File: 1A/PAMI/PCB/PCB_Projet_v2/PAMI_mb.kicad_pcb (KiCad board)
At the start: 4 copper layers, 66.5 x 58.4 mm, 107 parts, among them J1 Conn_02x20_Odd_Even, J10 Conn_01x04, J11 Conn_01x04, J12 Conn_01x04, J13 Conn_01x04, J2 Conn_01x03, J3 Conn_ST_STDC14, J4 Battery, J5 Charge, J6 Stop, J8 173010542, J9 Conn_01x04, SW1 SW_Push_SPDT, SW2 RotaryEncoder_Switch, SW3 SW_Push, SW4 SW_Push, SW5 SW_Push, SW6 SW_Push, U1 STM32G431KBTx, U2 LT1076CR-PBF, U3 AZ1117CH2-3.3TRG1, U4 TMC2225-SA-T, U5 TMC2225-SA-T

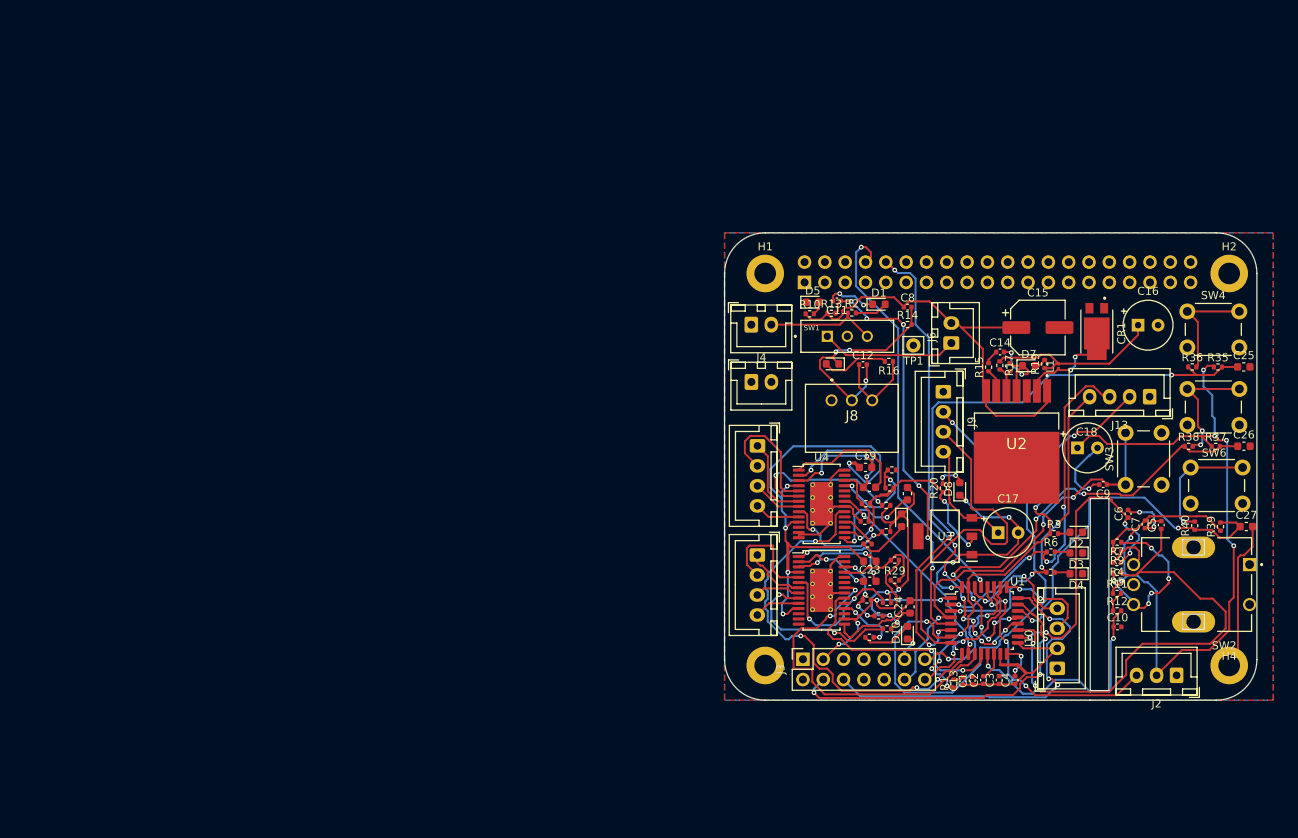
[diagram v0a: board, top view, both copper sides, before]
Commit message: update pcb
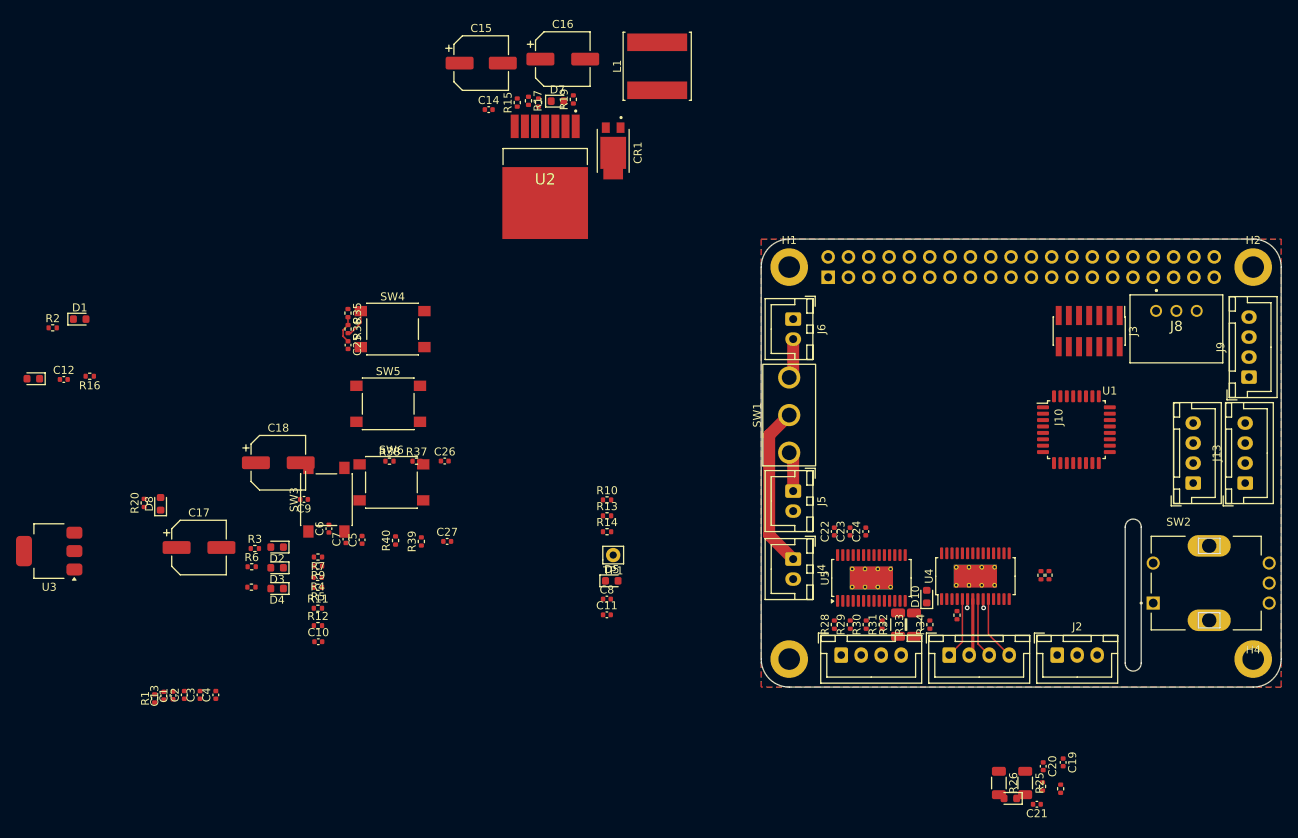
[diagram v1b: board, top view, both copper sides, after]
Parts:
- C16, C17, C18: footprint Capacitor_THT:CP_Radial_Tantal_D6.0mm_P2.50mm -> Capacitor_SMD:CP_Elec_6.3x5.4
- C19, C20, C21, C22, C23, C24, C25, C26, C27: footprint Capacitor_SMD:C_0603_1608Metric -> Capacitor_SMD:C_0402_1005Metric
- J3: footprint Connector_PinSocket_2.54mm:PinSocket_2x07_P2.54mm_Vertical -> Connector_PinHeader_1.27mm:PinHeader_2x07_P1.27mm_Vertical_SMD
- L1: footprint Inductor_SMD:L_0201_0603Metric -> Inductor_SMD:L_Changjiang_FNR8065S
- R25, R26, R32, R33: footprint Resistor_SMD:R_0402_1005Metric -> Resistor_SMD:R_1206_3216Metric
- SW1: footprint MINI_SPDT_SW:SW_MINI-SPDT-SW -> Library:472121010111
- SW3, SW4, SW5, SW6: footprint Button_Switch_THT:SW_PUSH_6mm -> Button_Switch_SMD:SW_Push_1P1T_NO_6x6mm_H9.5mm
- U3: footprint AZ1117_CH2:SOT230P700X180-4N -> Package_TO_SOT_SMD:SOT-223-3_TabPin2
- moved U3 112.0 mm to (37.5, 85.5)
- moved C25 112.0 mm to (74.9, 59.8), turned to -90 degrees
- moved R35 109.0 mm to (74.8, 55.8), turned to -90 degrees
- moved R36 105.6 mm to (74.9, 57.8), turned to -90 degrees
- moved C1 99.9 mm to (53.0, 103.5)
- moved C13 99.9 mm to (51.8, 103.6)
- moved C2 99.9 mm to (54.4, 103.5)
- moved C26 99.9 mm to (86.9, 74.2)
- moved C3 99.9 mm to (56.4, 103.5)
- moved R11 99.9 mm to (71.1, 92.6)
- moved R39 99.9 mm to (84.0, 84.3)
- moved R40 99.9 mm to (80.8, 84.2)
- moved C10 99.9 mm to (71.1, 96.8)
- moved C12 99.9 mm to (39.3, 64.0)
- moved C17 99.9 mm to (56.2, 85.1)
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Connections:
- J11 pad 1: /TMC2225/OA1 -> /TMC2225/OA2
- J11 pad 2: /TMC2225/OA2 -> /TMC2225/OA1
- J12 pad 1: /TMC2226/OA1 -> /TMC2226/OA2
- J12 pad 2: /TMC2226/OA2 -> /TMC2226/OA1
- J4 pad 1: GND -> /V_BAT
- J4 pad 2: /V_BAT -> GND
- J5 pad 1: GND -> /V_CHARGE
- J5 pad 2: /V_CHARGE -> GND
- J6 pad 1: Net-(J6-Pin_1) -> VCC
- J6 pad 2: VCC -> Net-(J6-Pin_2)
- SW1 pad 1: Net-(J6-Pin_1) -> Net-(J6-Pin_2)
- U1 pad 10: /PWM_MOTOR_L_TIM2_CH1 -> /PWM_MOTOR_R_TIM3_CH1
- U1 pad 11: /PWM_MOTOR_R_TIM3_CH1 -> /PWM_MOTOR_L_TIM2_CH1
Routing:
- net +3.3V: track 195.6 -> 0.00 mm, vias 14 -> 0
- net GND: track 180.6 -> 0.00 mm, vias 21 -> 0
- net VCC: track 115.3 -> 0.00 mm, vias 5 -> 0
- net /PA1_USR_BTN_0: track 79.0 -> 3.53 mm, vias 4 -> 0
- net /LIDAR_LP_TX: track 69.6 -> 0.00 mm, vias 2 -> 0
- net /ENCODEUR_B: track 62.4 -> 0.00 mm, vias 2 -> 0
- net /RASPBERRY_PI_RX: track 61.0 -> 0.00 mm, vias 10 -> 0
- net /PA11_USR_BTN_1: track 59.9 -> 0.00 mm, vias 8 -> 0
- net /PB8-BOOT0_LED0: track 55.5 -> 0.00 mm, vias 6 -> 0
- net /DIR_MOTOR_L: track 53.4 -> 0.00 mm, vias 4 -> 0
- net /NRST: track 52.4 -> 0.00 mm, vias 3 -> 0
- net /RASPBERRY_PI_TX: track 52.2 -> 0.00 mm, vias 2 -> 0
- net /ADC_BATT: track 52.0 -> 0.00 mm, vias 6 -> 0
- net /SWCLK: track 46.5 -> 0.00 mm, vias 3 -> 0
- net /PA12_USR_BTN_2: track 45.2 -> 0.00 mm, vias 2 -> 0
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- removed copper zone on In1.Cu, net +3.3V
- removed copper zone on In1.Cu, net +5.1V
- removed copper zone on In1.Cu, net +5V
- removed copper zone on In1.Cu, net /V_BAT
- removed copper zone on In1.Cu, net /V_CHARGE
- removed copper zone on In1.Cu, net VCC
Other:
- board size 66.5 x 58.4 mm -> 65 x 56 mm
